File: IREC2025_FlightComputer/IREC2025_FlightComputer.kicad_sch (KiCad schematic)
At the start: 68 parts, among them J1 Molex Microfit, J2 BOOT0, J4 Conn_02x03_Counter_Clockwise, Q1 SI7232DN-T1-GE3, Q2 SI7232DN-T1-GE3, U1 STM32U575VGTx, U2 NRVB120VLSFT1G, U4 NRVB120VLSFT1G, U5 LP5912Q3.3DRVRQ1, U8 TPS62153, U9 SN74HCT125DR, X1 1XXD32000MBA

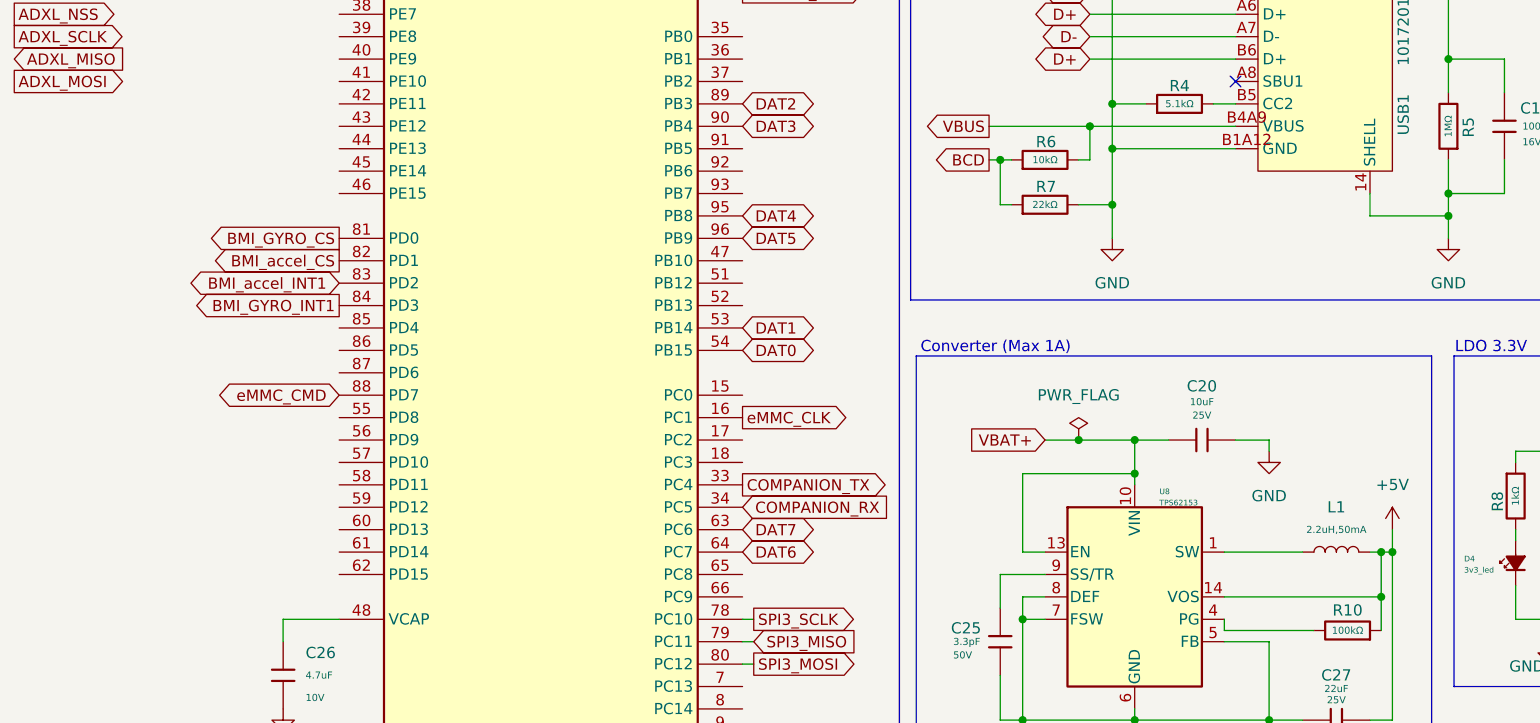
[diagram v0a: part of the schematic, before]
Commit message: update idk
25/3/2025
starting to take shape (i guess)
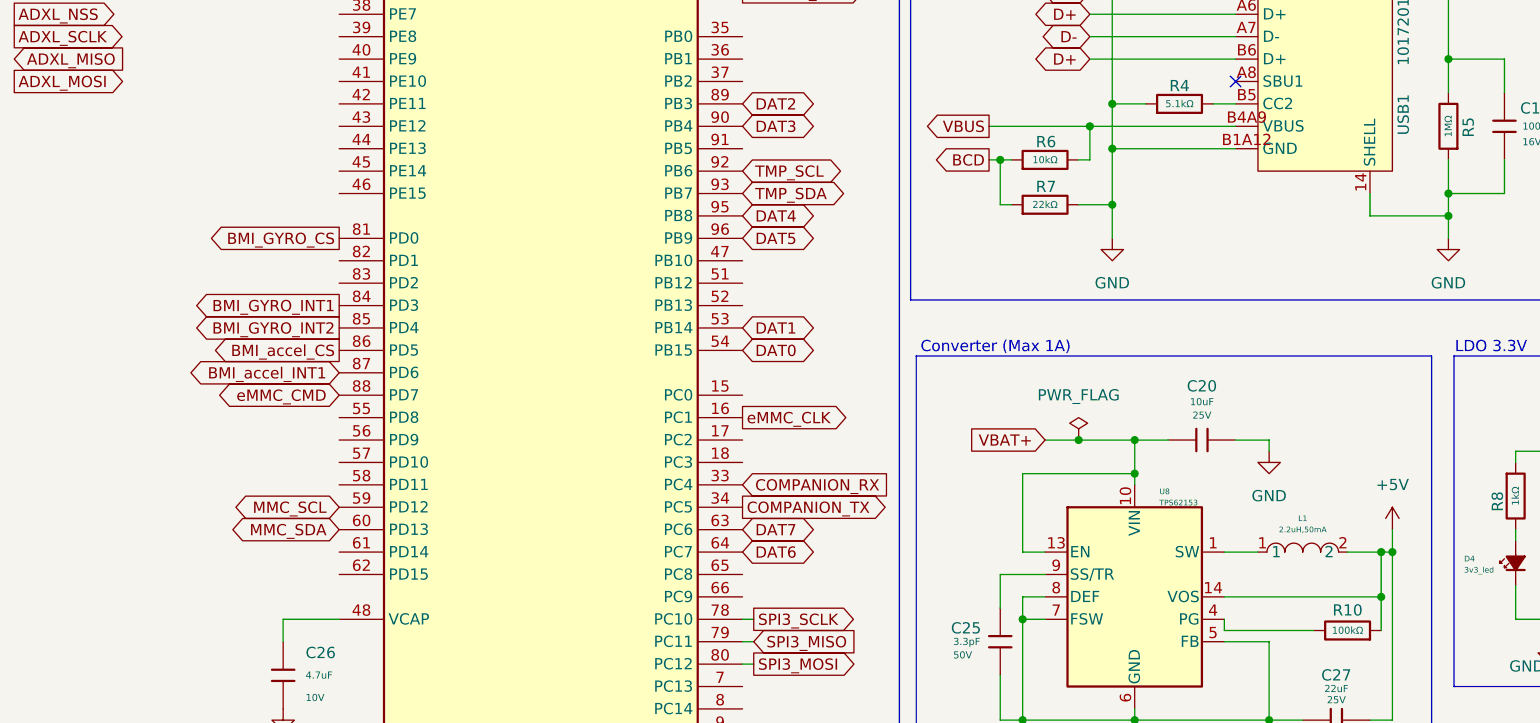
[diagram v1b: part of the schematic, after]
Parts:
- removed L1: 2.2uH,50mA, PCM_JLCPCB:L_0805, symbol PCM_JLCPCB-Inductors:2.2uH,50mA
- added L1: 2.2uH,50mA, EasyEDA:IND-SMD_L4.0-W4.0_XFL4020-102MEB, symbol EasyEDA:XFL4020-472MEC
- D3: footprint EasyEDA:SMA_L4.4-W2.6-LS5.0-RD -> GNSS:DIOM7959X262N
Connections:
- net +5V: now also L1.2
- net BMI_accel_CS: now also U1.86 (PD5); no longer U1.82 (PD1)
- net BMI_accel_INT1: now also U1.87 (PD6); no longer U1.83 (PD2)
- net COMPANION_RX: now also U1.33 (PC4); no longer U1.34 (PC5)
- net COMPANION_TX: now also U1.34 (PC5); no longer U1.33 (PC4)
- net at U8.1 (SW), U8.2 (SW), U8.3 (SW): now also L1.1
- net MMC_SCL: now reaches U1.59 (PD12)
- net MMC_SDA: now reaches U1.60 (PD13)
- net BMI_GYRO_INT2: now reaches U1.85 (PD4)
- net TMP_SCL: now reaches U1.92 (PB6)
- net TMP_SDA: now reaches U1.93 (PB7)

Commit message: checkpoint
before the great layout change
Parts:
- removed C19, C22: 100nF, PCM_JLCPCB:C_0402, symbol PCM_JLCPCB-Capacitors:0402,100nF
- removed C23: RVT1E101M0607, EasyEDA:CAP-SMD_BD6.3-L6.6-W6.6-LS7.2-R-RD, symbol EasyEDA:RVT1E101M0607
- removed C25: 3.3pF, PCM_JLCPCB:C_0402, symbol PCM_JLCPCB-Capacitors:0402,3.3pF
- removed C27: 22uF, PCM_JLCPCB:C_0805, symbol PCM_JLCPCB-Capacitors:0805,22uF
- removed C28: 100uF, PCM_JLCPCB:C_CASE-B-3528-21(mm), symbol PCM_JLCPCB-Capacitors:CASE-B-3528-21(mm),100uF
- removed D4: 3v3_led, LED_SMD:LED_0805_2012Metric, symbol Device:LED_Small_Filled
- removed Pyro_C1: Molex Microfit, Connector_Molex:Molex_Micro-Fit_3.0_43650-0215_1x02_P3.00mm_Vertical, symbol Connector:Conn_01x02_Socket
- removed Q2: SI7232DN-T1-GE3, EasyEDA:POWER-1212-8_L3.3-W3.3-P0.66-LS3.3-BL, symbol EasyEDA:SI7232DN-T1-GE3
- removed R11: 3.3kΩ, PCM_JLCPCB:R_0402, symbol PCM_JLCPCB-Resistors:0402,3.3kΩ
- removed R5: 1MΩ, PCM_JLCPCB:R_0402, symbol PCM_JLCPCB-Resistors:0402,1MΩ
- removed R6: 10kΩ, PCM_JLCPCB:R_0402, symbol PCM_JLCPCB-Resistors:0402,10kΩ
- removed R7: 22kΩ, PCM_JLCPCB:R_0402, symbol PCM_JLCPCB-Resistors:0402,22kΩ
- removed R8: 1kΩ, PCM_JLCPCB:R_0805, symbol PCM_JLCPCB-Resistors:0805,1kΩ
- added C22: 100nF, PCM_JLCPCB:C_0402, symbol Device:C_Small
- added C23: 22uF, PCM_JLCPCB:C_0603, symbol PCM_JLCPCB-Capacitors:0603,22uF
- added C24: 10uF, PCM_JLCPCB:C_0805, symbol PCM_JLCPCB-Capacitors:1206,10uF
- added C25: GJM1555C1H3R3BB01D, EasyEDA:C0402, symbol EasyEDA:GJM1555C1H3R3BB01D
- added C28, C74: 100uF, EasyEDA:CAP-SMD_L3.2-W1.6, symbol EasyEDA:T520A107M006ATE070
- added C70: 100nF, PCM_JLCPCB:C_0402, symbol PCM_JLCPCB-Capacitors:1206,100nF
- added H1, H2, H3, H4: MountingHole_Pad, MountingHole:MountingHole_3.2mm_M3_DIN965_Pad, symbol Mechanical:MountingHole_Pad
- added SERVO2: Conn_01x03_Pin, Connector_Molex:Molex_Micro-Fit_3.0_43650-0315_1x03_P3.00mm_Vertical, symbol Connector:Conn_01x03_Pin
- C1: name (none) -> CC0402JRNPO9BN101
- C10, C13, C17, C2: name (none) -> GRM155R71H104KE14D
- C12, C3: name (none) -> GRM155R70J105KA12D
- C14: name (none) -> C0402C103K4RECTU
- C18: name (none) -> GRM155R61A106ME11D
- C20: footprint PCM_JLCPCB:C_0603 -> PCM_JLCPCB:C_0805; Temperature Coefficient X5R -> X7R; namw (none) -> CL21B106KOQNNNE
- C21: footprint PCM_JLCPCB:C_0402 -> PCM_JLCPCB:C_0603; Name (none) -> CL10B225KP8NNNC; Temperature Coefficient X5R -> X7R
- C26: footprint PCM_JLCPCB:C_0402 -> PCM_JLCPCB:C_0603; Temperature Coefficient X5R -> X7R; name (none) -> GRM188Z71A475ME15D
- C4: footprint PCM_JLCPCB:C_0402 -> PCM_JLCPCB:C_0805
- L1: namw (none) -> 74437349047
- R1: name (none) -> RC0402JR-0710KL
- R10: name (none) -> RC0402JR-07100KL
- R12: Name (none) -> RC0402FR-07470RL x 4
- R16, R17: name (none) -> ERA-2AEB332X
- R2: name (none) -> RC0402FR-0747KL
- R3, R4: Name (none) -> ERA-2AEB512X
- R38, R9: Name (none) -> RC0402JR-0710KL
- renumbered Pyro_A1 to Pyro_CH1, Pyro_B1 to Pyro_CH2, PWM1 to SERVO1
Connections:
- net +3V3 is gone; now on net +3.3V: J2.1 (Pin_1), R38.1
- net PYRO_C is gone; now on net SERVO_A: U9.8 (3Y)
- net VREF+ is gone; now on net +3.3VA: C3.1, U1.21 (VREF+)
- net +3.3V: no longer U9.14 (VCC)
- net +5V: now also U9.14 (VCC), C23.2, C28.1, SERVO2.1 (Pin_1)
- net ADXL_MISO: now also U1.17 (PC2)
- net ADXL_MOSI: now also U1.18 (PC3)
- net ADXL_NSS: now also U1.51 (PB12)
- net ADXL_SCLK: now also U1.47 (PB10)
- net BAT_LEVEL: now also U1.97 (PE0)
- net BMI_GYRO_INT1: now also U1.83 (PD2); no longer U1.84 (PD3)
- net BMI_GYRO_INT2: now also U1.84 (PD3); no longer U1.85 (PD4)
- net BMI_accel_CS: now also U1.85 (PD4); no longer U1.86 (PD5)
- net BMI_accel_INT1: now also U1.86 (PD5); no longer U1.87 (PD6)
- net DAT0: now also U1.53 (PB14); no longer U1.54 (PB15)
- net DAT1: now also U1.54 (PB15); no longer U1.53 (PB14)
- net DAT6: now also U1.63 (PC6); no longer U1.64 (PC7)
- net DAT7: now also U1.64 (PC7); no longer U1.63 (PC6)
- net GND: now also USB1.13 (SHELL), C22.2, C23.1, C24.2, C25.1, C28.2, C70.2, C74.2, H1.1, H2.1, H3.1, H4.1, SERVO2.2 (Pin_2)
- net PWM_A: now also U1.2 (PE3)
- net PWM_B: now also U1.3 (PE4)
- net PWM_C: now also U1.4 (PE5)
- net PWM_D: now also U1.5 (PE6)
- net SERVO_A: no longer U9.11 (4Y)
- net VBAT+: now also C24.1, C70.1
- net nRST: now also C22.1
- net at U8.9 (SS/TR): now also C25.2
- net at U2.1 (K), U4.1 (K), U5.4 (EN)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: now also C74.1
- net BUZZER: now reaches U1.40 (PE9)
- net ADXL_INT2: now reaches U1.41 (PE10)
- net ADXL_INT1: now reaches U1.42 (PE11)
- net LoRa_RST: now reaches U1.43 (PE12)
- net GNSS_SAFEBOOT: now reaches U1.44 (PE13)
- net BUSY: now reaches U1.52 (PB13)
- net LORA_DIO3: now reaches U1.55 (PD8)
- net RST_n: now reaches U1.58 (PD11)
- net ANT_SW: now reaches U1.69 (PA10)
- net TMP_ALERT: now reaches U1.91 (PB5)
- new net BMI_accel_INT2: U1.87 (PD6)
- new net SERVO_B: SERVO2.3 (Pin_3), U9.11 (4Y)
- no-connect marks 9 -> 27
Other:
- note added: "CL21B106KOQNNNE"
- note added: "Companion"
- note added: "GRM155R70J105KA12D"
- note added: "GRM155R71H104KE14D"
- note added: "Pyro connectors (COTS EAGLE and COTS TENDER)"
- note added: "Pyro_CH1 (COTS TENDER)"
- note added: "Pyro_CH2 (EAGLE)"
- note added: "SERVO_CH1 (DODO-separation)"
- note added: "SERVO_CH1 (DODO_SEPARATION)"
- note added: "SERVO_CH2 (LEASH)"
- note added: "Servo Connectors (SRAD DODO and SRAD LEASH)"
- note removed: "Pyro connectors"
- note removed: "Servo Connector"
- note removed: "Testing point"
- moved on the sheet: SERVO1
